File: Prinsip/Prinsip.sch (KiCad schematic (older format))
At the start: 9 parts

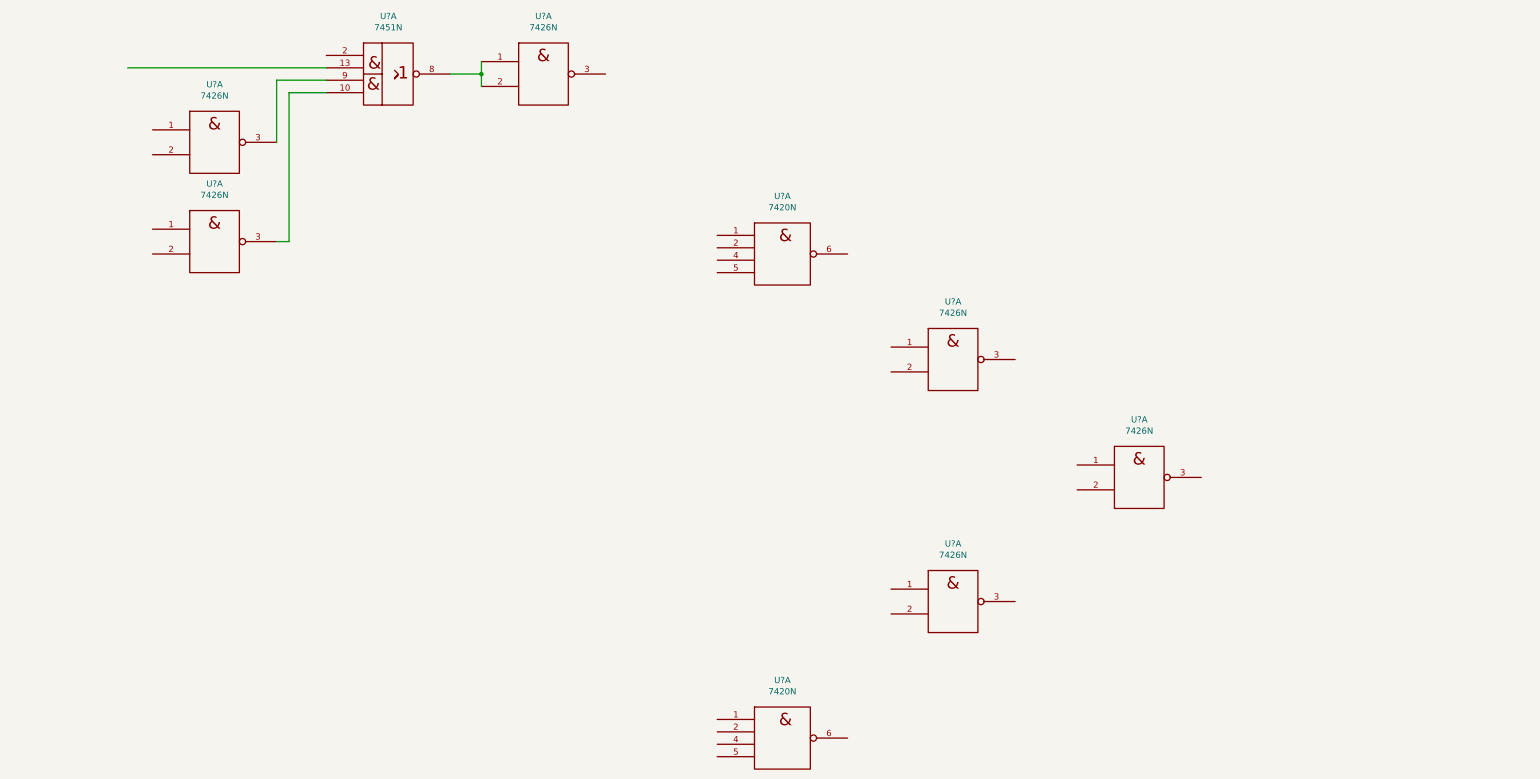
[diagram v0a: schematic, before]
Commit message: Optimized
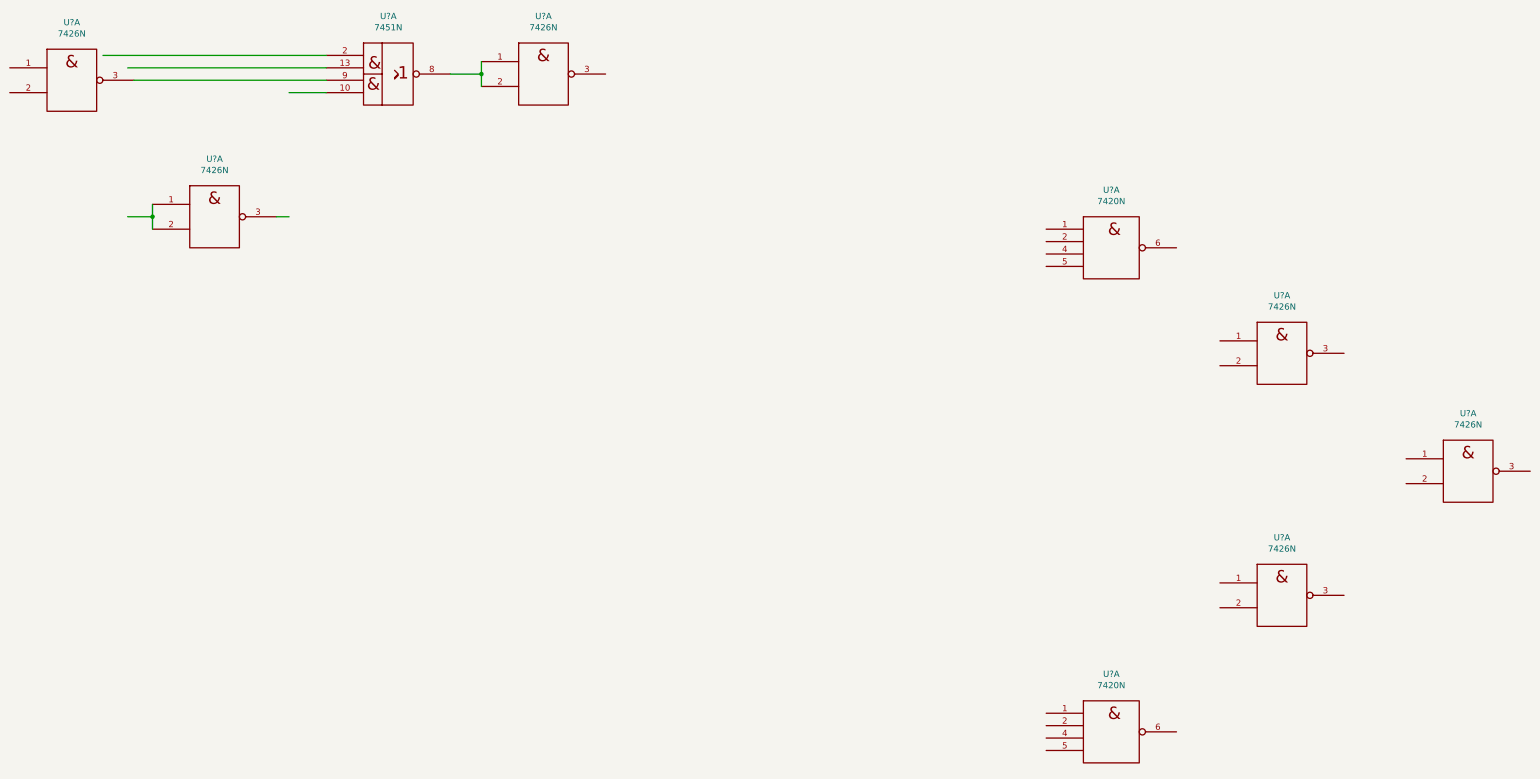
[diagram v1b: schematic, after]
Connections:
- wire segments 9 -> 11
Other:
- moved on the sheet: U?A
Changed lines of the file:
@@
 L Prinsip:7420N U?
 U 1 1 61669E61
-P 8100 3100
-F 0 "U?" H 8075 3566 50  0000 C CNN
-F 1 "7420N" H 8075 3475 50  0000 C CNN
-F 2 "" H 8100 3250 50  0001 C CNN
-F 3 "" H 8100 3250 50  0001 C CNN
-	1    8100 3100
+P 10750 3050
+F 0 "U?" H 10725 3516 50  0000 C CNN
+F 1 "7420N" H 10725 3425 50  0000 C CNN
+F 2 "" H 10750 3200 50  0001 C CNN
+F 3 "" H 10750 3200 50  0001 C CNN
+	1    10750 3050
 	1    0    0    -1
 $EndComp
@@
 L Prinsip:7420N U?
 U 1 1 6166CDF9
-P 8100 7000
-F 0 "U?" H 8075 7466 50  0000 C CNN
-F 1 "7420N" H 8075 7375 50  0000 C CNN
-F 2 "" H 8100 7150 50  0001 C CNN
-F 3 "" H 8100 7150 50  0001 C CNN
-	1    8100 7000
+P 10750 6950
+F 0 "U?" H 10725 7416 50  0000 C CNN
+F 1 "7420N" H 10725 7325 50  0000 C CNN
+F 2 "" H 10750 7100 50  0001 C CNN
+F 3 "" H 10750 7100 50  0001 C CNN
+	1    10750 6950
 	1    0    0    -1
 $EndComp
@@
 L Prinsip:7426N U?
 U 1 1 6166FCF7
-P 9450 3950
-F 0 "U?" H 9450 4416 50  0000 C CNN
-F 1 "7426N" H 9450 4325 50  0000 C CNN
-F 2 "" H 9450 4100 50  0001 C CNN
-F 3 "" H 9450 4100 50  0001 C CNN
-	1    9450 3950
+P 12100 3900
+F 0 "U?" H 12100 4366 50  0000 C CNN
+F 1 "7426N" H 12100 4275 50  0000 C CNN
+F 2 "" H 12100 4050 50  0001 C CNN
+F 3 "" H 12100 4050 50  0001 C CNN
+	1    12100 3900
 	1    0    0    -1
 $EndComp
@@
 L Prinsip:7426N U?
 U 1 1 61671269
-P 9450 5900
-F 0 "U?" H 9450 6366 50  0000 C CNN
-F 1 "7426N" H 9450 6275 50  0000 C CNN
-F 2 "" H 9450 6050 50  0001 C CNN
-F 3 "" H 9450 6050 50  0001 C CNN
-	1    9450 5900
+P 12100 5850
+F 0 "U?" H 12100 6316 50  0000 C CNN
+F 1 "7426N" H 12100 6225 50  0000 C CNN
+F 2 "" H 12100 6000 50  0001 C CNN
+F 3 "" H 12100 6000 50  0001 C CNN
+	1    12100 5850
 	1    0    0    -1
 $EndComp
@@
 L Prinsip:7426N U?
 U 1 1 61671C84
-P 10950 4900
-F 0 "U?" H 10950 5366 50  0000 C CNN
-F 1 "7426N" H 10950 5275 50  0000 C CNN
-F 2 "" H 10950 5050 50  0001 C CNN
-F 3 "" H 10950 5050 50  0001 C CNN
-	1    10950 4900
-	1    0    0    -1
-$EndComp
-$Comp
-L Prinsip:7426N U?
-U 1 1 6166AF0B
-P 3500 3000
-F 0 "U?" H 3500 3466 50  0000 C CNN
-F 1 "7426N" H 3500 3375 50  0000 C CNN
-F 2 "" H 3500 3150 50  0001 C CNN
-F 3 "" H 3500 3150 50  0001 C CNN
-	1    3500 3000
+P 13600 4850
+F 0 "U?" H 13600 5316 50  0000 C CNN
+F 1 "7426N" H 13600 5225 50  0000 C CNN
+F 2 "" H 13600 5000 50  0001 C CNN
+F 3 "" H 13600 5000 50  0001 C CNN
+	1    13600 4850
 	1    0    0    -1
 $EndComp
@@
 L Prinsip:7426N U?
 U 1 1 6166A9DA
-P 3500 2200
-F 0 "U?" H 3500 2666 50  0000 C CNN
-F 1 "7426N" H 3500 2575 50  0000 C CNN
-F 2 "" H 3500 2350 50  0001 C CNN
-F 3 "" H 3500 2350 50  0001 C CNN
-	1    3500 2200
+P 2350 1700
+F 0 "U?" H 2350 2166 50  0000 C CNN
+F 1 "7426N" H 2350 2075 50  0000 C CNN
+F 2 "" H 2350 1850 50  0001 C CNN
+F 3 "" H 2350 1850 50  0001 C CNN
+	1    2350 1700
 	1    0    0    -1
 $EndComp
 Wire Wire Line
-	4400 1700 4000 1700
-Wire Wire Line
-	4000 1700 4000 2200
-Wire Wire Line
 	4400 1800 4100 1800
-Wire Wire Line
-	4100 1800 4100 3000
-Wire Wire Line
-	4100 3000 4000 3000
 $Comp
 L Prinsip:7426N U?
@@
 Wire Wire Line
 	5650 1650 5650 1750
+Wire Wire Line
+	4400 1500 2600 1500
+Wire Wire Line
+	2850 1700 4400 1700
+Wire Wire Line
+	4100 2800 4000 2800
+$Comp
+L Prinsip:7426N U?
+U 1 1 6166AF0B
+P 3500 2800
+F 0 "U?" H 3500 3266 50  0000 C CNN
+F 1 "7426N" H 3500 3175 50  0000 C CNN
+F 2 "" H 3500 2950 50  0001 C CNN
+F 3 "" H 3500 2950 50  0001 C CNN
+	1    3500 2800
+	1    0    0    -1
+$EndComp
+Wire Wire Line
+	3000 2700 3000 2800
+Wire Wire Line
+	2800 2800 3000 2800
+Connection ~ 3000 2800
+Wire Wire Line
+	3000 2800 3000 2900
 $EndSCHEMATC
